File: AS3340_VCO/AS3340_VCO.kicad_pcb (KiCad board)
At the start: 2 copper layers, 71.1 x 43.2 mm, 69 parts, among them J1 CV_In, J12 Conn_01x10, J2 Waveform_Out, U1 AS3340, U2 TL071, U4 TL071, U5 LM13700, U6 TL072

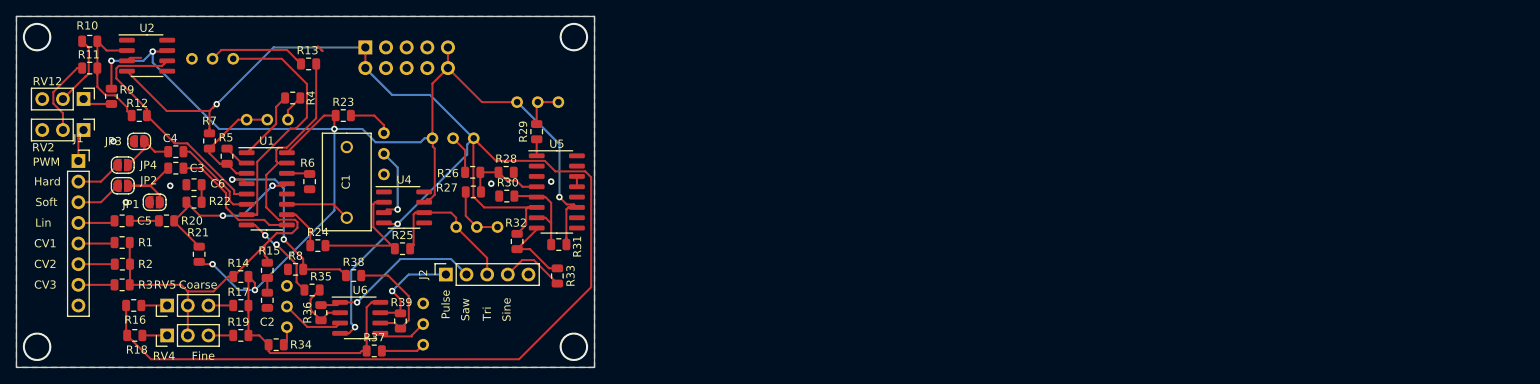
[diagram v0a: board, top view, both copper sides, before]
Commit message: AS3340_VCO rev 2 AS3310_ADSR rev 1 AS3320_VCF rev 1 AS3360_VCA rev 1 ER_Bus_Board rev 1
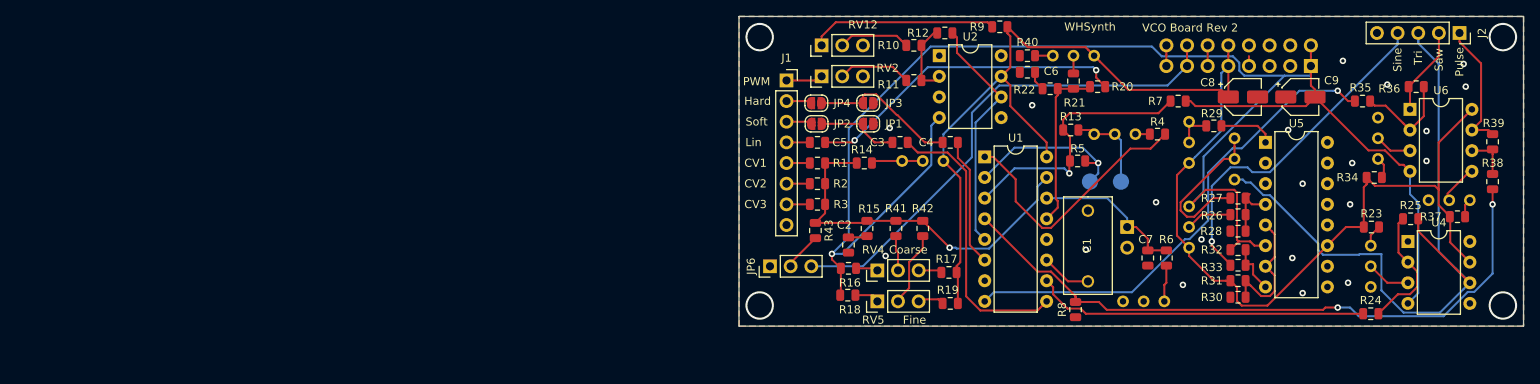
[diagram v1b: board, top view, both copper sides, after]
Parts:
- removed J12: Conn_01x10, Connector_IDC:IDC-Header_2x05_P2.54mm_Vertical
- added C7: 560pF, Capacitor_SMD:C_0805_2012Metric, F.Cu at (190.0, 93.2)
- added C8: 10uF, Capacitor_SMD:CP_Elec_4x3, F.Cu at (201.7, 73.4)
- added C9: 10uF, Capacitor_SMD:CP_Elec_4x3, F.Cu at (208.8, 73.4)
- added J3: Power, Connector_IDC:IDC-Header_2x08_P2.54mm_Vertical, B.Cu at (210.1, 69.6)
- added JP5: Jumper, Connector_PinHeader_2.54mm:PinHeader_1x02_P2.54mm_Vertical, B.Cu at (187.5, 89.4)
- added JP6: Jumper_3_Open, Connector_PinHeader_2.54mm:PinHeader_1x03_P2.54mm_Vertical, F.Cu at (143.5, 94.2)
- added R40: 47K, Resistor_SMD:R_0805_2012Metric, F.Cu at (175.2, 68.3)
- added R41: 100K, Resistor_SMD:R_0805_2012Metric, F.Cu at (159.0, 89.6)
- added R42: 1M, Resistor_SMD:R_0805_2012Metric, F.Cu at (162.3, 89.6)
- added R43: 100K 0.05%, Resistor_SMD:R_0805_2012Metric, F.Cu at (149.1, 89.8)
- added RV13: 100K, Potentiometer_THT:Potentiometer_Bourns_3296W_Vertical, B.Cu at (164.8, 81.3)
- added RV14: 10K, Potentiometer_THT:Potentiometer_Bourns_3296W_Vertical, B.Cu at (183.4, 68.3)
- added TP1: TestPoint, TestPoint:TestPoint_Pad_D2.0mm, B.Cu at (182.9, 83.8)
- added TP2: TestPoint, TestPoint:TestPoint_Pad_D2.0mm, B.Cu at (186.7, 83.8)
- R1, R2, R3: value 100K -> 100K 0.05%
- R13: value 1M -> 5.6K
- R14: value 360K -> 200K
- R21: value 1.5M -> 1.2M
- R4: value 24K -> 18K
- R6: value 1.8K -> 470
- RV1: value 10K -> 5K
- RV3: value 20K -> 1K
- U1, U5: footprint Package_SO:SOIC-16_3.9x9.9mm_P1.27mm -> Package_DIP:DIP-16_W7.62mm
- U2, U4, U6: footprint Package_SO:SOIC-8_3.9x4.9mm_P1.27mm -> Package_DIP:DIP-8_W7.62mm
- moved R38 140.6 mm to (232.4, 83.8), turned to 90 degrees
- moved R36 137.6 mm to (223.0, 72.1), turned to 180 degrees
- moved R34 136.7 mm to (217.9, 83.3)
- moved R39 136.2 mm to (232.4, 78.9)
- moved RV10 135.8 mm to (218.3, 81.0)
- moved R37 134.3 mm to (228.1, 88.1)
- moved U6 131.7 mm to (222.2, 74.9)
- moved R35 131.3 mm to (216.4, 73.9)
- moved RV11 130.0 mm to (229.6, 86.1), turned to 0 degrees
- moved R24 129.8 mm to (217.4, 100.1)
- moved J2 128.2 mm to (228.3, 65.5), turned to 270 degrees
- moved R23 127.2 mm to (217.5, 89.4)
- moved R25 124.1 mm to (222.3, 88.4)
- moved U4 123.6 mm to (222.0, 91.2)
- moved RV3 123.3 mm to (192.0, 98.6), turned to 0 degrees
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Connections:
- R13 pad 1: /Input Conditioning/CV -> /Vee
- R14 pad 1: +12V -> Net-(R14-Pad1)
- R21 pad 2: +12V -> Net-(R21-Pad2)
- R6 pad 1: GNDREF -> Net-(R6-Pad1)
- RV1 pad 2: /Vee -> Net-(R13-Pad2)
- RV1 pad 3: /Vee -> Net-(R13-Pad2)
- RV3 pad 1: GNDREF -> Net-(R6-Pad1)
- RV3 pad 2: Net-(R13-Pad2) -> GNDREF
- RV3 pad 3: /Input Conditioning/HFT -> GNDREF
- RV4 pad 2: /Input Conditioning/CV -> Net-(R41-Pad2)
- RV5 pad 2: /Input Conditioning/CV -> Net-(R42-Pad2)
- U1 pad 7: /Input Conditioning/HFT -> Net-(U1-Pad7)
- U2 pad 1: (no net) -> Net-(U2-Pad1)
- U2 pad 5: (no net) -> Net-(U2-Pad5)
- U2 pad 8: (no net) -> Net-(U2-Pad8)
- U4 pad 1: (no net) -> Net-(U4-Pad1)
- U4 pad 5: (no net) -> Net-(U4-Pad5)
- U4 pad 8: (no net) -> Net-(U4-Pad8)
- U5 pad 10: (no net) -> Net-(U5-Pad10)
- U5 pad 12: (no net) -> Net-(U5-Pad12)
- U5 pad 15: (no net) -> Net-(U5-Pad15)
- U5 pad 16: (no net) -> Net-(U5-Pad16)
- U5 pad 2: (no net) -> Net-(U5-Pad2)
- U5 pad 9: (no net) -> Net-(U5-Pad9)
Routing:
- net /Output Conditioning/TRI: track 18.6 -> 88.4 mm
- net /ER_CV: track 0.00 -> 62.2 mm
- net /Output Conditioning/RAW_PULSE: track 25.3 -> 80.7 mm
- net /Output Conditioning/RAW_SAW: track 11.7 -> 60.2 mm, vias 2 -> 1
- net Net-(C5-Pad1): track 3.59 -> 39.8 mm, vias 0 -> 2
- net /Output Conditioning/RAW_TRI: track 5.63 -> 41.1 mm
- net /Output Conditioning/SINE: track 8.03 -> 42.5 mm, vias 0 -> 1
- net /Input Conditioning/HFT: track 30.7 -> 0.00 mm
- net Net-(R4-Pad2): track 8.74 -> 32.2 mm
- net Net-(R9-Pad1): track 3.76 -> 23.0 mm
- net /Vee: track 15.4 -> 34.1 mm, vias 0 -> 1
- net /Input Conditioning/SOFT_SYNC: track 16.8 -> 35.2 mm
- net /Input Conditioning/CV: track 64.5 -> 46.4 mm, vias 0 -> 1
- net Net-(R5-Pad2): track 3.15 -> 20.7 mm, vias 0 -> 1
- net Net-(C7-Pad2): track 2.83 -> 18.9 mm
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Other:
- board size 71.1 x 43.2 mm -> 96.5 x 38.1 mm
- board text added: "Pulse Offset"
- board text added: "Ref Pitch"
- board text added: "Refind"
- board text added: "Saw Offset"
- board text added: "Tempco Adj"
- board text added: "Tri Offset"
- board text added: "VCO Board Rev 2"
- board text added: "WHSynth"
- board text removed: "HFT"
- board text removed: "Pulse Level"
- board text removed: "Saw Level"
- board text removed: "Tri Level"
